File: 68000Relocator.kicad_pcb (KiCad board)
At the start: 2 copper layers, 97.5 x 97.4 mm, 2 parts, among them U1 68000D, U2 68000D

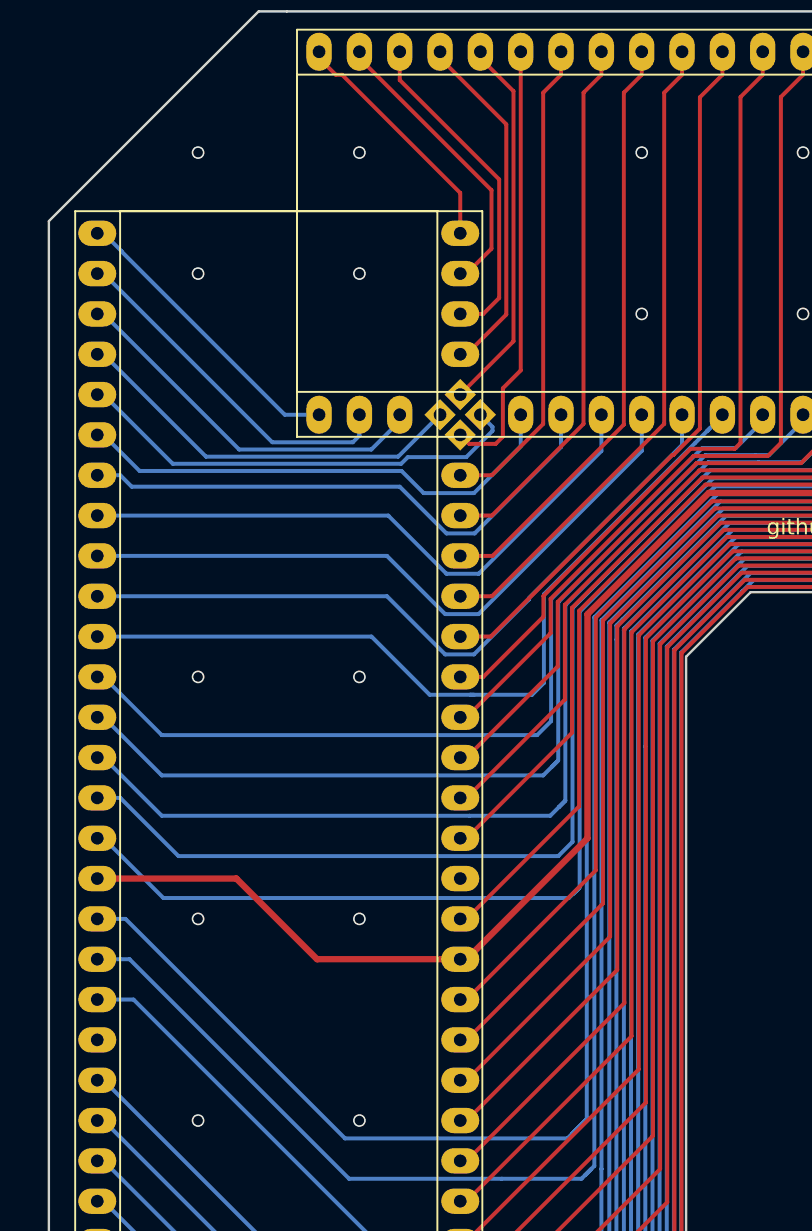
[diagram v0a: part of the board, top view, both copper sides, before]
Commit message: Fix tracks
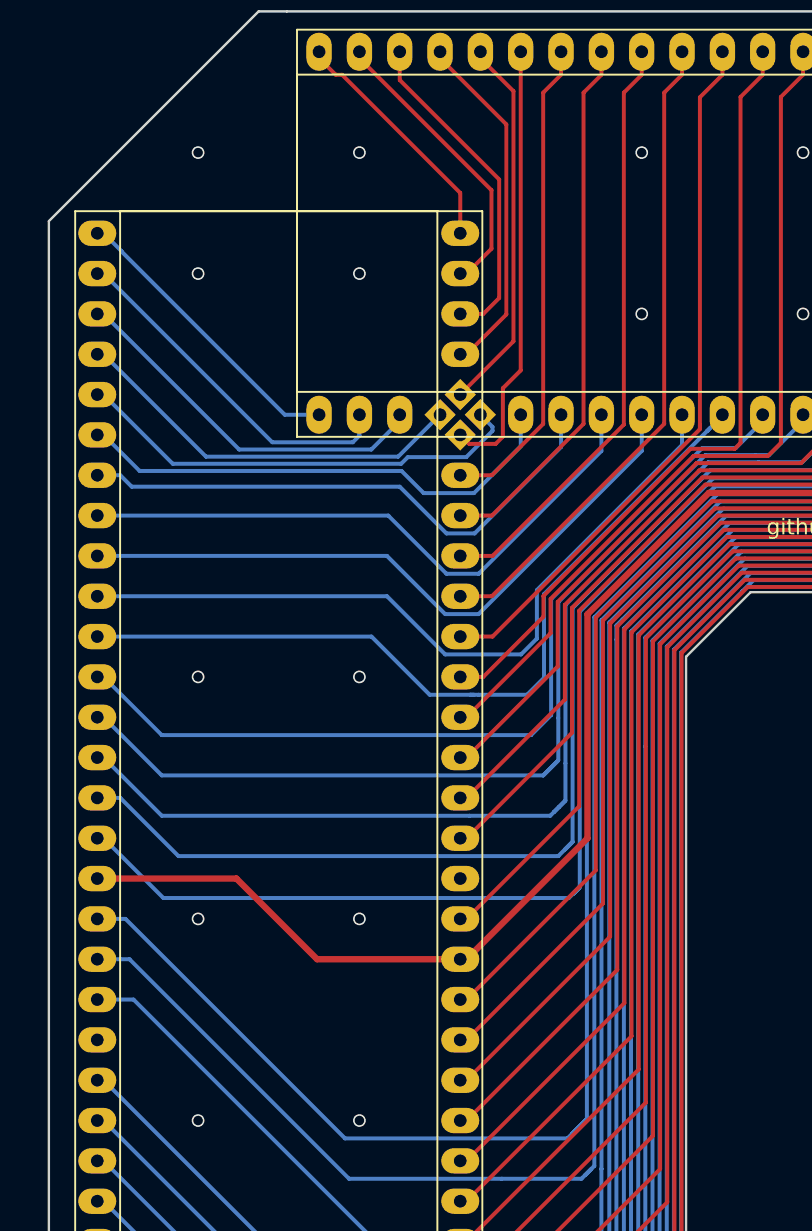
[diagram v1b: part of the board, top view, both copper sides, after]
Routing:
- net /A14: track 45.9 -> 47.7 mm
- net /A21: track 102.9 -> 103.8 mm
- net /A17: track 62.0 -> 62.8 mm
- net /A19: track 71.4 -> 72.1 mm
- net /A20: track 78.6 -> 79.2 mm
